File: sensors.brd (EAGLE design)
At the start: 80 x 80 mm, 5 parts

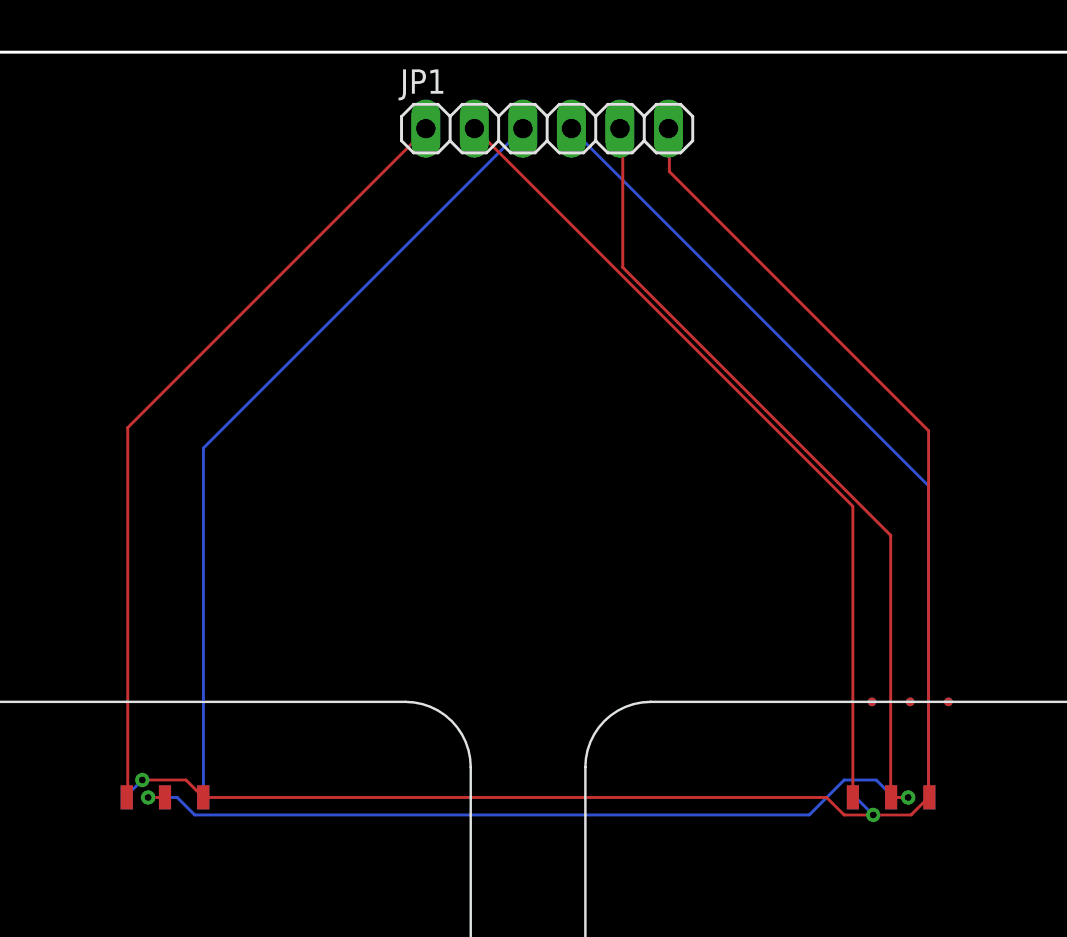
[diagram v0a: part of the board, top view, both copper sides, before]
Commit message: updated
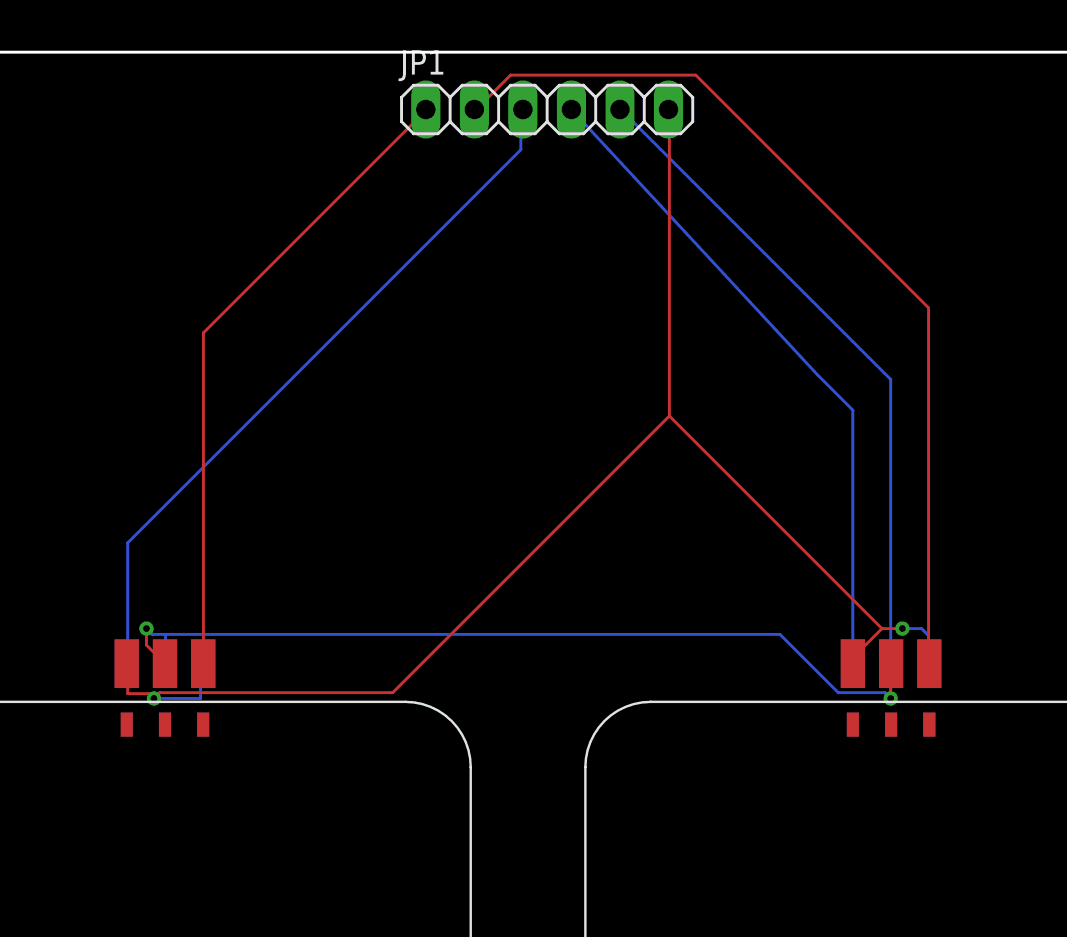
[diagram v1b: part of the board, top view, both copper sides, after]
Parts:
- added PAD1, PAD10, PAD11, PAD12, PAD2, PAD3, PAD4, PAD5, PAD6, PAD7, PAD8, PAD9: WIREPADSMD1,27-254, wirepad:SMD1,27-2,54
- moved JP1 1.00 mm to (41.0, 77.0)
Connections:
- net 3.3V: now also PAD12.1, PAD3.1, PAD6.1, PAD9.1; no longer U$1.P$3, U$2.P$3, U$3.P$3, U$4.P$3
- net GND: now also PAD11.1, PAD2.1, PAD5.1, PAD8.1; no longer U$1.P$2, U$2.P$2, U$3.P$2, U$4.P$2
- net GPIO34: now also PAD4.1; no longer U$2.P$1
- net GPIO35: now also PAD7.1; no longer U$3.P$1
- net GPIO36: now also PAD1.1; no longer U$1.P$1
- net GPIO39: now also PAD10.1; no longer U$4.P$1
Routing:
- net GPIO39: track 42.7 -> 34.8 mm
- net GPIO36: track 41.5 -> 33.8 mm
- net 3.3V: track 85.6 -> 78.9 mm
- net GPIO34: track 43.2 -> 48.2 mm
- net GPIO35: track 41.9 -> 37.6 mm
- net GND: track 84.0 -> 82.5 mm
